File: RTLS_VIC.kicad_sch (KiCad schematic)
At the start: 35 parts, among them J1 Conn_01x02_Pin, SW1 TS-1187A-B-A-B, U1 STM32WLE5CBUx, U3 HXY4612S, U4 TPS63900DSKR, X1 Q24FA20H0021700

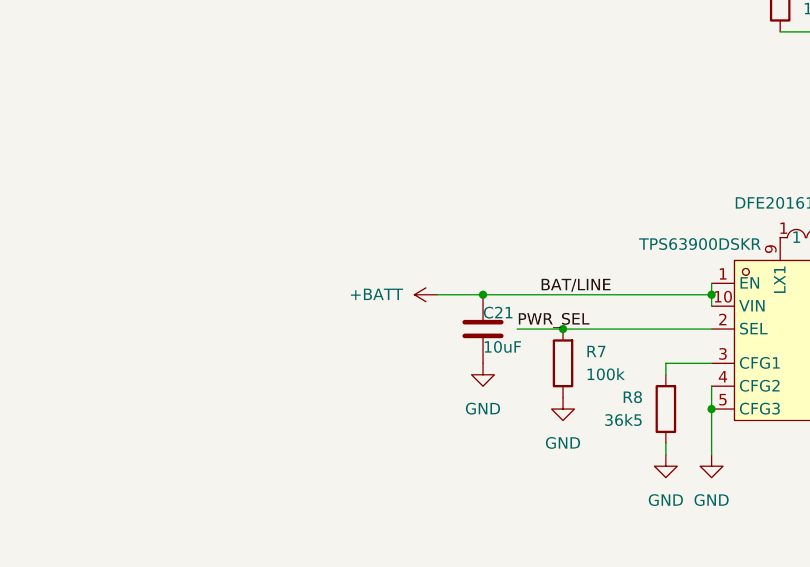
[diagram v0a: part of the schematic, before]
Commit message: add notes
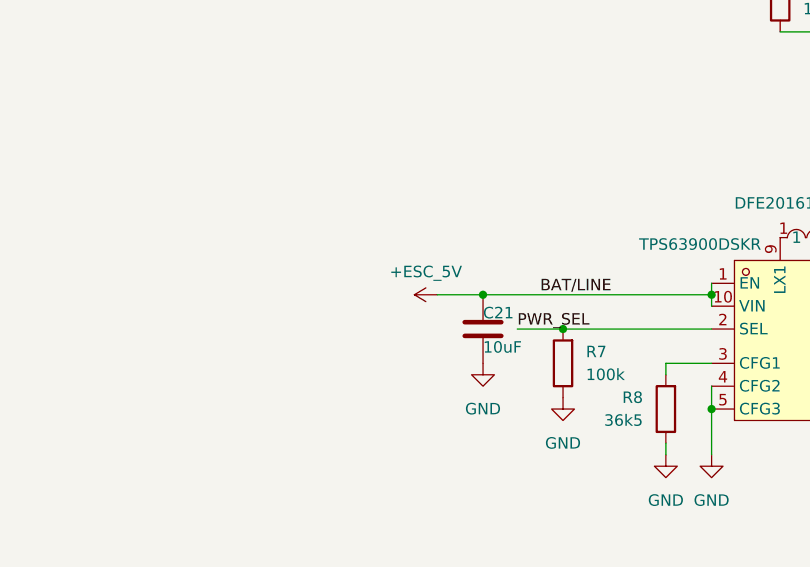
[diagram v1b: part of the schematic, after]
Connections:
- net +BATT: no longer C21.1, U4.1 (EN), U4.10 (VIN)
- new net +ESC_5V: C21.1, U4.1 (EN), U4.10 (VIN)
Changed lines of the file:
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@@
 			)
 		)
-		(property "Value" "+BATT"
-			(at 184.15 134.6199 90)
+		(property "Value" "+ESC_5V"
+			(at 186.69 132.08 90)
 			(effects
 				(font
 					(size 1.27 1.27)
 				)
-				(justify left)
 			)
 		)

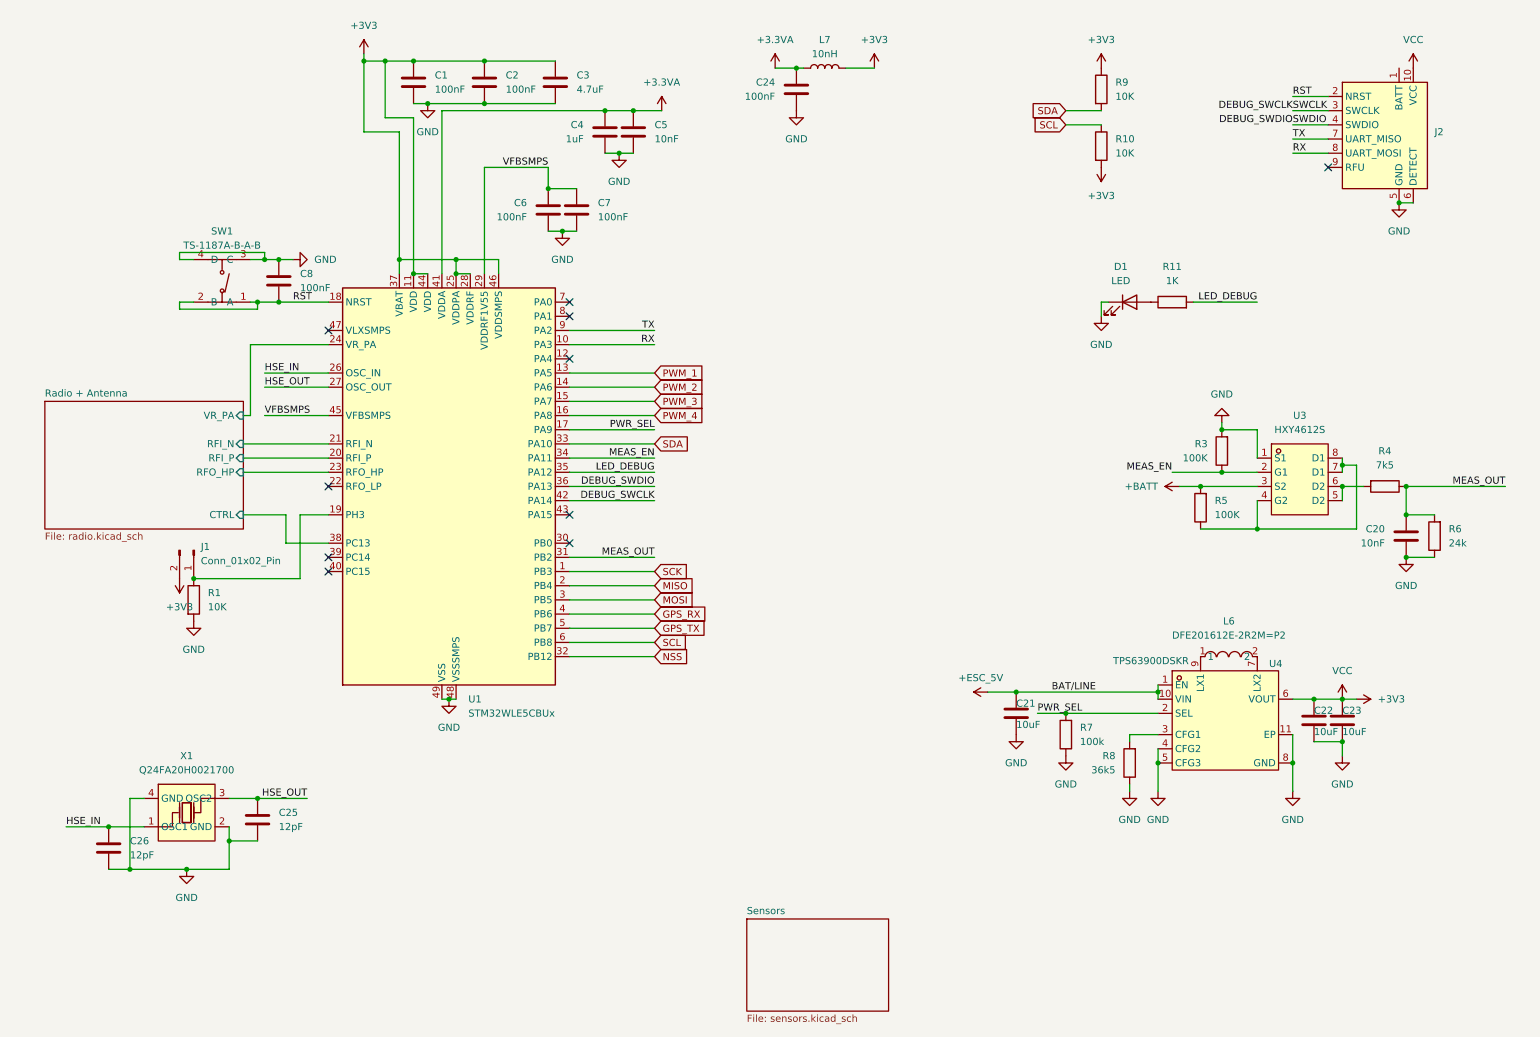
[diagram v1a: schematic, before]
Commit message: major overhaul
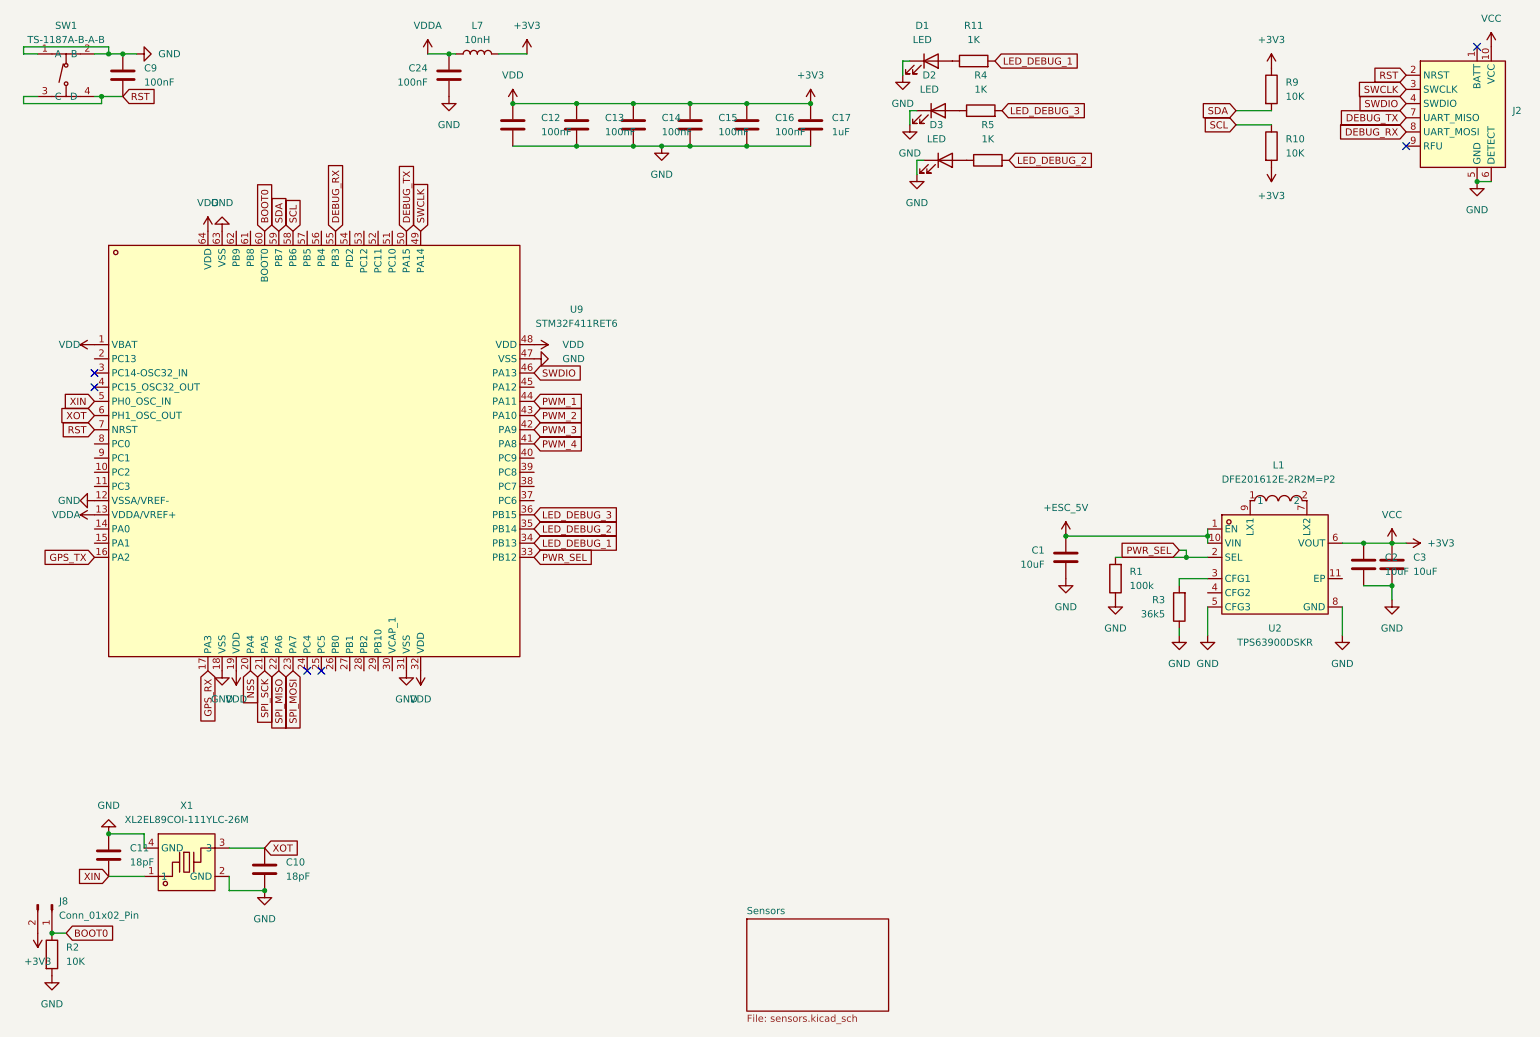
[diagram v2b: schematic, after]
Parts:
- removed C20, C5: 10nF, Capacitor_SMD:C_0402_1005Metric, symbol Device:C
- removed C21, C22, C23: 10uF, Capacitor_SMD:C_0402_1005Metric, symbol Device:C
- removed C25, C26: 12pF, Capacitor_SMD:C_0402_1005Metric, symbol Device:C
- removed C4: 1uF, Capacitor_SMD:C_0402_1005Metric, symbol Device:C
- removed C6, C7, C8: 100nF, Capacitor_SMD:C_0402_1005Metric, symbol Device:C
- removed J1: Conn_01x02_Pin, Connector_PinHeader_2.54mm:PinHeader_1x02_P2.54mm_Vertical, symbol Connector:Conn_01x02_Pin
- removed L6: DFE201612E-2R2M=P2, dfe2016:L0806, symbol dfe2016:DFE201612E-2R2M=P2
- removed R6: 24k, Resistor_SMD:R_0603_1608Metric, symbol Device:R
- removed R7: 100k, Resistor_SMD:R_0603_1608Metric, symbol Device:R
- removed R8: 36k5, Resistor_SMD:R_0603_1608Metric, symbol Device:R
- removed SW1: TS-1187A-B-A-B, ts-1187a-b-a-b:SW-SMD_4P-L5.1-W5.1-P3.70-LS6.5-TL_H1.5, symbol ts-1187a-b-a-b:TS-1187A-B-A-B
- removed U1: STM32WLE5CBUx, Package_DFN_QFN:QFN-48-1EP_7x7mm_P0.5mm_EP5.6x5.6mm, symbol MCU_ST_STM32WL:STM32WLE5CBUx
- removed U3: HXY4612S, hxy4612s:SOP-8_L4.9-W3.9-P1.27-LS6.0-BL, symbol hxy4612s:HXY4612S
- removed U4: TPS63900DSKR, tps63900:WSON-10_L2.5-W2.5-W0.50-TL-EP, symbol tps63900:TPS63900DSKR
- removed X1: Q24FA20H0021700, q24:CRYSTAL-SMD_4P-L2.5-W2.0-BL, symbol q24:Q24FA20H0021700
- added C10, C11: 18pF, Capacitor_SMD:C_0402_1005Metric, symbol Device:C
- added C12, C13, C14, C15, C16, C9: 100nF, Capacitor_SMD:C_0402_1005Metric, symbol Device:C
- added C17: 1uF, Capacitor_SMD:C_0402_1005Metric, symbol Device:C
- added D2, D3: LED, LED_SMD:LED_0603_1608Metric, symbol Device:LED
- added J8: Conn_01x02_Pin, Connector_PinHeader_2.54mm:PinHeader_1x02_P2.54mm_Vertical, symbol Connector:Conn_01x02_Pin
- added L1: DFE201612E-2R2M=P2, lib:L0806, symbol lib:DFE201612E-2R2M=P2
- added R2: 10K, Resistor_SMD:R_0603_1608Metric, symbol Device:R
- added SW1: TS-1187A-B-A-B, lib:SW-SMD_4P-L5.1-W5.1-P3.70-LS6.5-TL_H1.5, symbol lib:TS-1187A-B-A-B
- added U2: TPS63900DSKR, lib:WSON-10_L2.5-W2.5-W0.50-TL-EP, symbol lib:TPS63900DSKR
- added U9: STM32F411RET6, lib:LQFP-64_L10.0-W10.0-P0.50-LS12.0-BL, symbol lib:STM32F411RET6
- added X1: XL2EL89COI-111YLC-26M, lib:CRYSTAL-SMD_4P-L3.2-W2.5-BL_SIT8008BI, symbol lib:XL2EL89COI-111YLC-26M
- C1, C2: value 100nF -> 10uF; LCSC (none) -> C15525
- C3: value 4.7uF -> 10uF; LCSC (none) -> C15525
- R1: value 10K -> 100k; LCSC (none) -> C25803
- R3: value 100K -> 36k5; LCSC (none) -> C23029
- R4: value 7k5 -> 1K
- R5: value 100K -> 1K
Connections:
- net MEAS_EN is gone; now on net GND: R3.1
- net +3V3: now also C12.1, C13.1, C14.1, C15.1, C16.1, C17.1, J8.2 (Pin_2), U2.6 (VOUT), U9.1 (VBAT), U9.19 (VDD), U9.32 (VDD), U9.48 (VDD), U9.64 (VDD); no longer C1.1
- net +ESC_5V: now also C1.1, U2.1 (EN), U2.10 (VIN)
- net GND: now also R1.1, C10.2, C11.1, C12.2, C13.2, C14.2, C15.2, C16.2, C17.2, C9.1, D2.1 (K), D3.1 (K), R2.2, SW1.1 (A), SW1.2 (B), U2.5 (CFG3), U2.8 (GND), U9.12 (VSSA/VREF-), U9.18 (VSS), U9.31 (VSS), U9.47 (VSS), U9.63 (VSS), X1.2 (GND), X1.4 (GND); no longer R1.2, R3.2
- net GPS_RX: now also U9.17 (PA3)
- net GPS_TX: now also U9.16 (PA2)
- net NSS: now also U9.20 (PA4)
- net PWM_1: now also U9.44 (PA11)
- net PWM_2: now also U9.43 (PA10)
- net PWM_3: now also U9.42 (PA9)
- net PWM_4: now also U9.41 (PA8)
- net PWR_SEL: now also R1.2, U2.2 (SEL), U9.33 (PB12)
- net RST: now also C9.2, SW1.3 (C), SW1.4 (D), U9.7 (NRST)
- net SCL: now also U9.58 (PB6)
- net SDA: now also U9.59 (PB7)
- net LED_DEBUG_3: now reaches R4.2
- net LED_DEBUG_3: now also U9.36 (PB15)
- net at R5.1: now also D3.2 (A)
- net +3.3VA renamed VDDA
- net VDDA: now also U9.13 (VDDA/VREF+)
- net +BATT renamed LED_DEBUG_2
- net LED_DEBUG_2: now also U9.35 (PB14)
- net DEBUG_SWCLK renamed SWCLK
- net SWCLK: now also U9.49 (PA14)
- net DEBUG_SWDIO renamed SWDIO
- net SWDIO: now also U9.46 (PA13)
- net LED_DEBUG renamed LED_DEBUG_1
- net LED_DEBUG_1: now also U9.34 (PB13)
- net MEAS_OUT: no longer names the net of R4.1
- net MEAS_OUT: now also D2.2 (A)
- net RX renamed DEBUG_RX
- net DEBUG_RX: now also U9.55 (PB3)
- net TX renamed DEBUG_TX
- net DEBUG_TX: now also U9.50 (PA15)
- new net: R3.2, U2.3 (CFG1)
- new net: L1.2, U2.7 (LX2)
- new net: L1.1, U2.9 (LX1)
- new net BOOT0: J8.1 (Pin_1), R2.1, U9.60 (BOOT0)
- new net SPI_MISO: U9.22 (PA6)
- new net SPI_MOSI: U9.23 (PA7)
- new net SPI_SCK: U9.21 (PA5)
- new net XIN: C11.2, U9.5 (PH0_OSC_IN), X1.1
- new net XOT: C10.1, U9.6 (PH1_OSC_OUT), X1.3
- no-connect marks 10 -> 6
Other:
- removed sheet Radio + Antenna
- moved on the sheet: C24, D1, J2, L7, R10, R11, R9
